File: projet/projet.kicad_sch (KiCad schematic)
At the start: 19 parts, among them J301 EMB_P3.81_1x02_VERTICAL, J302 EMB_P3.81_1x04_VERTICAL, Q301 MOS P 20V 2A, U301 Raspberry-Pi-Pico_Linked

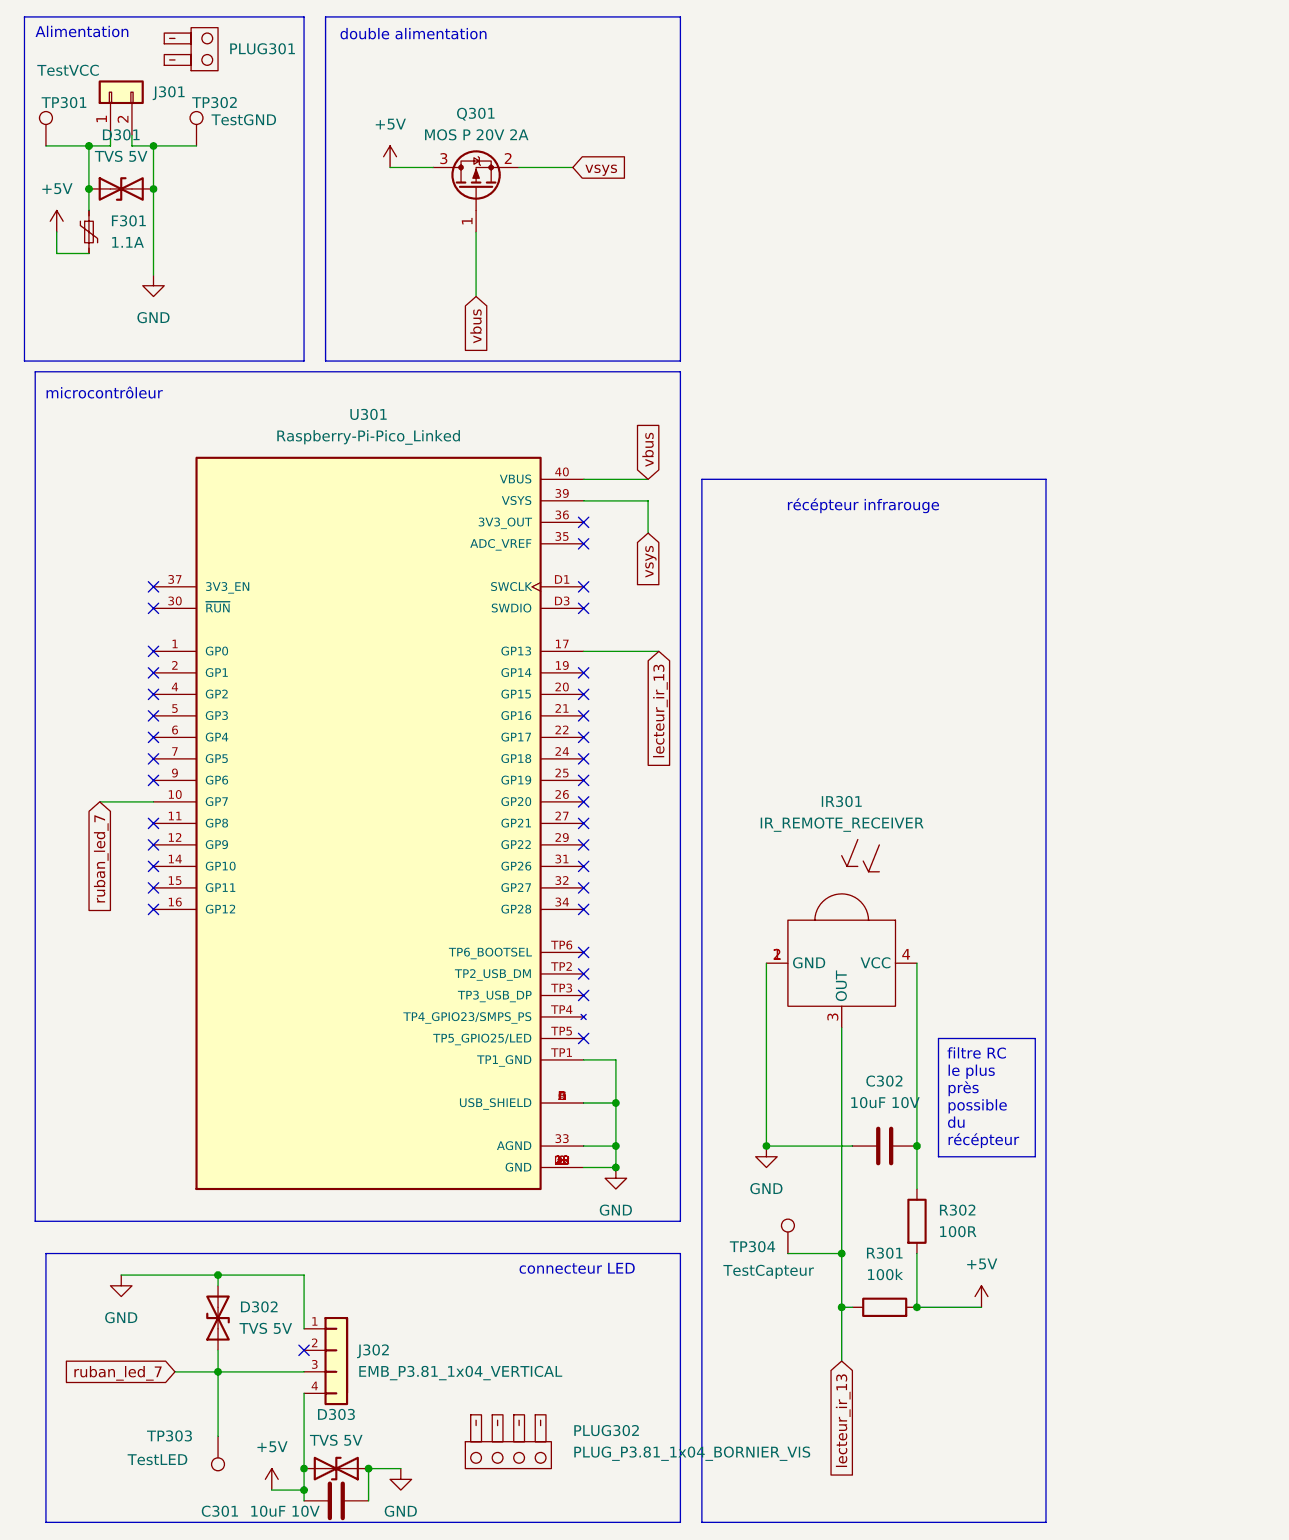
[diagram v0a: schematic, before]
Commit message: Dernière modifs avant vérif externes
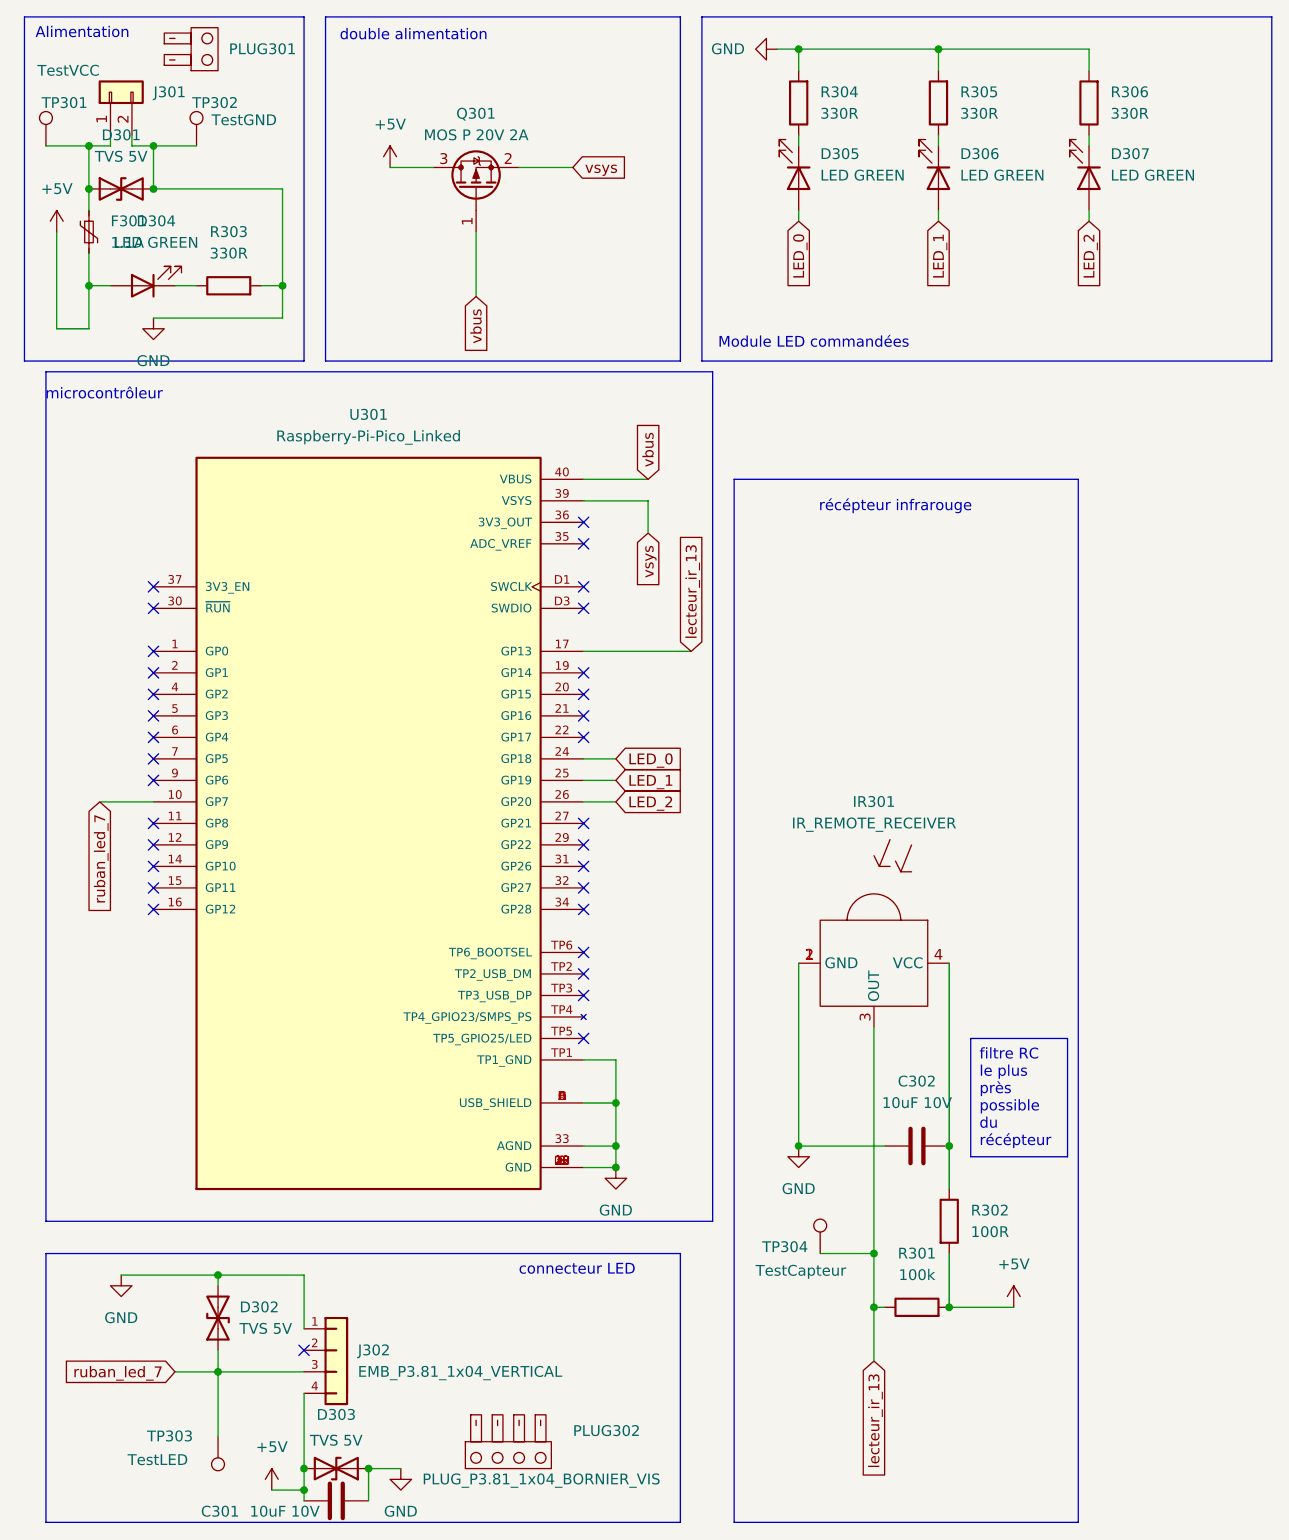
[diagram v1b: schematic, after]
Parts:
- added D304, D305, D306, D307: LED GREEN, codium_Leds:LED0805, symbol codium_Leds:LED_0805_Green
- added R303, R304, R305, R306: 330R, codium_Basics:R0603, symbol codium_Resistors:R_0603_330R
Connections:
- net +5V: now also D304.2 (A)
- net GND: now also R303.2, R304.2, R305.2, R306.2
- net LED_0: now reaches U301.24 (GP18)
- net LED_0: now also D305.2 (A)
- net LED_1: now reaches U301.25 (GP19)
- net LED_1: now also D306.2 (A)
- net LED_2: now reaches U301.26 (GP20)
- net LED_2: now also D307.2 (A)
- new net: D304.1 (K), R303.1
- new net: D306.1 (K), R305.1
- new net: D305.1 (K), R304.1
- new net: D307.1 (K), R306.1
- no-connect marks 35 -> 32
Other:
- note added: "Module LED commandées"
- moved on the sheet: C302, IR301, R301, R302, TP304
